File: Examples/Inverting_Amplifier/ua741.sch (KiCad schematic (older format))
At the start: 7 parts, among them U1 PORT

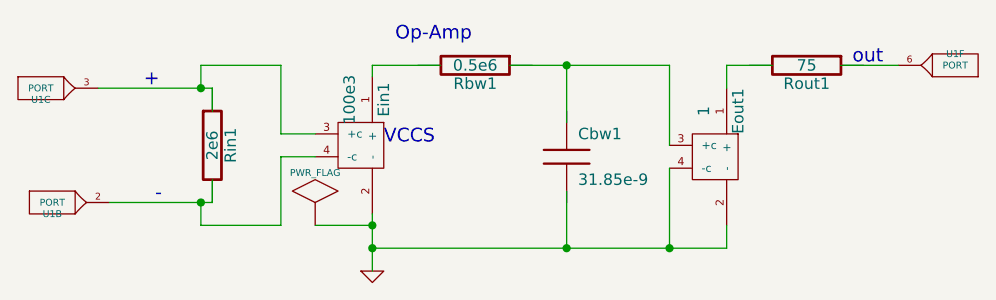
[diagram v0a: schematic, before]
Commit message: Modified Example
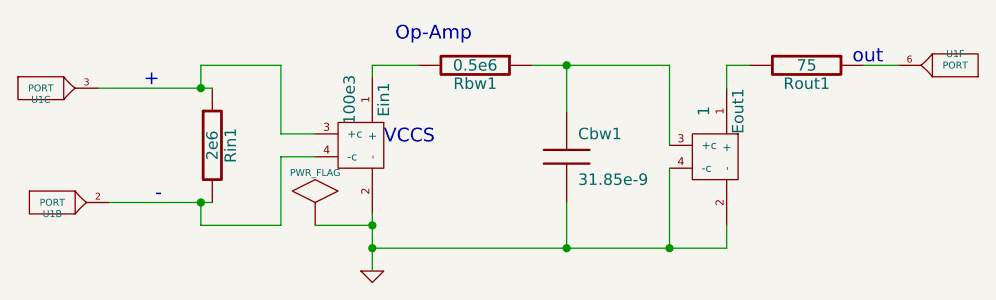
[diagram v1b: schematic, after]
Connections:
- wire segments 26 -> 24
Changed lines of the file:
@@
-EESchema Schematic File Version 2
+EESchema Schematic File Version 2  date Wednesday 19 December 2012 10:15:16 AM IST
 LIBS:power
 LIBS:device
@@
 LIBS:analogXSpice
 LIBS:ua741-cache
-EELAYER 25 0
+EELAYER 25  0
 EELAYER END
-$Descr A4 11693 8268
+$Descr A4 11700 8267
 encoding utf-8
 Sheet 1 1
@@
 F 0 "U1" H 6250 2450 30  0000 C CNN
 F 1 "PORT" H 6250 2500 30  0000 C CNN
-F 2 "" H 6250 2500 60  0001 C CNN
-F 3 "" H 6250 2500 60  0001 C CNN
 	6    6250 2500
 	-1   0    0    1
@@
 F 0 "U1" H 2300 3050 30  0000 C CNN
 F 1 "PORT" H 2300 3100 30  0000 C CNN
-F 2 "" H 2300 3100 60  0001 C CNN
-F 3 "" H 2300 3100 60  0001 C CNN
 	2    2300 3100
 	1    0    0    -1
@@
 F 0 "U1" H 2250 2550 30  0000 C CNN
 F 1 "PORT" H 2250 2600 30  0000 C CNN
-F 2 "" H 2250 2600 60  0001 C CNN
-F 3 "" H 2250 2600 60  0001 C CNN
 	3    2250 2600
 	1    0    0    -1
 $EndComp
+Connection ~ 3700 3200
+Wire Wire Line
+	3450 3200 3700 3200
+Connection ~ 5000 3300
+Wire Wire Line
+	3700 3300 5250 3300
+Wire Wire Line
+	5250 3300 5250 3200
+Connection ~ 4550 3300
+Wire Wire Line
+	5000 3300 5000 2950
+Connection ~ 3700 3300
+Wire Wire Line
+	4550 3300 4550 3100
+Wire Wire Line
+	3900 2500 3700 2500
+Wire Wire Line
+	3700 2500 3700 2550
+Wire Wire Line
+	3450 2900 3300 2900
+Wire Wire Line
+	3300 2900 3300 3200
+Wire Wire Line
+	3300 3200 2950 3200
+Connection ~ 2950 3100
+Wire Wire Line
+	2950 3200 2950 3100
+Wire Wire Line
+	3000 2600 2500 2600
+Wire Wire Line
+	2550 3100 3000 3100
+Wire Wire Line
+	2950 2600 2950 2500
+Connection ~ 2950 2600
+Wire Wire Line
+	2950 2500 3300 2500
+Wire Wire Line
+	3300 2500 3300 2800
+Wire Wire Line
+	3300 2800 3450 2800
+Wire Wire Line
+	3700 3150 3700 3400
+Wire Wire Line
+	4550 2500 4550 2700
+Wire Wire Line
+	4400 2500 5000 2500
+Wire Wire Line
+	5000 2500 5000 2850
+Connection ~ 4550 2500
+Wire Wire Line
+	5250 2600 5250 2500
+Wire Wire Line
+	5250 2500 5350 2500
+Wire Wire Line
+	5850 2500 6000 2500
 $Comp
 L PWR_FLAG #FLG01
@@
 F 0 "#FLG01" H 3450 3470 30  0001 C CNN
 F 1 "PWR_FLAG" H 3450 3430 30  0000 C CNN
-F 2 "" H 3450 3200 60  0001 C CNN
-F 3 "" H 3450 3200 60  0001 C CNN
 	1    3450 3200
 	1    0    0    -1
@@
 F 0 "Rout1" V 5680 2500 50  0000 C CNN
 F 1 "75" V 5600 2500 50  0000 C CNN
-F 2 "" H 5600 2500 60  0001 C CNN
-F 3 "" H 5600 2500 60  0001 C CNN
 	1    5600 2500
 	0    1    1    0
@@
 F 0 "Eout1" H 5000 3000 50  0000 C CNN
 F 1 "1" H 5000 2850 50  0000 C CNN
-F 2 "" H 5200 2900 60  0001 C CNN
-F 3 "" H 5200 2900 60  0001 C CNN
 	1    5200 2900
 	0    1    1    0
@@
 F 0 "Cbw1" H 4600 3000 50  0000 L CNN
 F 1 "31.85e-9" H 4600 2800 50  0000 L CNN
-F 2 "" H 4550 2900 60  0001 C CNN
-F 3 "" H 4550 2900 60  0001 C CNN
 	1    4550 2900
 	1    0    0    -1
@@
 F 0 "Rbw1" V 4230 2500 50  0000 C CNN
 F 1 "0.5e6" V 4150 2500 50  0000 C CNN
-F 2 "" H 4150 2500 60  0001 C CNN
-F 3 "" H 4150 2500 60  0001 C CNN
 	1    4150 2500
 	0    1    1    0
@@
 F 0 "#PWR02" H 3700 3400 30  0001 C CNN
 F 1 "GND" H 3700 3330 30  0001 C CNN
-F 2 "" H 3700 3400 60  0001 C CNN
-F 3 "" H 3700 3400 60  0001 C CNN
 	1    3700 3400
 	1    0    0    -1
@@
 F 0 "Ein1" H 3450 2950 50  0000 C CNN
 F 1 "100e3" H 3450 2800 50  0000 C CNN
-F 2 "" H 3650 2850 60  0001 C CNN
-F 3 "" H 3650 2850 60  0001 C CNN
 	1    3650 2850
 	0    1    1    0
@@
 F 0 "Rin1" V 3080 2850 50  0000 C CNN
 F 1 "2e6" V 3000 2850 50  0000 C CNN
-F 2 "" H 3000 2850 60  0001 C CNN
-F 3 "" H 3000 2850 60  0001 C CNN
 	1    3000 2850
 	1    0    0    -1
 $EndComp
-Connection ~ 3700 3200
-Wire Wire Line
-	3450 3200 3700 3200
-Connection ~ 5000 3300
-Wire Wire Line
-	3700 3300 5250 3300
-Wire Wire Line
-	5250 3300 5250 3200
-Connection ~ 4550 3300
-Wire Wire Line
-	5000 3300 5000 2950
-Connection ~ 3700 3300
-Wire Wire Line
-	4550 3050 4550 3300
-Wire Wire Line
-	3700 2500 4000 2500
-Wire Wire Line
-	3700 2500 3700 2550
-Wire Wire Line
-	3450 2900 3300 2900
-Wire Wire Line
-	3300 2900 3300 3200
-Wire Wire Line
-	3300 3200 2950 3200
-Connection ~ 2950 3100
-Wire Wire Line
-	2950 3200 2950 3100
-Wire Wire Line
-	3000 2600 2500 2600
-Wire Wire Line
-	2550 3100 3000 3100
-Wire Wire Line
-	2950 2600 2950 2500
-Connection ~ 2950 2600
-Wire Wire Line
-	2950 2500 3300 2500
-Wire Wire Line
-	3300 2500 3300 2800
-Wire Wire Line
-	3300 2800 3450 2800
-Wire Wire Line
-	3700 3150 3700 3400
-Wire Wire Line
-	4550 2500 4550 2750
-Wire Wire Line
-	4300 2500 5000 2500
-Wire Wire Line
-	5000 2500 5000 2850
-Connection ~ 4550 2500
-Wire Wire Line
-	5250 2600 5250 2500
-Wire Wire Line
-	5250 2500 5450 2500
-Wire Wire Line
-	5750 2500 6000 2500
-Wire Wire Line
-	3000 3100 3000 3000
-Wire Wire Line
-	3000 2700 3000 2600
 $EndSCHEMATC
